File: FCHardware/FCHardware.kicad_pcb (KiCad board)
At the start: 2 copper layers, 39 x 39 mm, 51 parts, among them J2 JST-4pin, J3 JST-8pin, J4 UJ20-C-H-G-SMT-2A-P16-TR, U1 ICM-42688-P, U2 STM32F405RGTx, U3 USBLC6-2SC6, U4 AP2112K-3.3, U5 TPSM63603

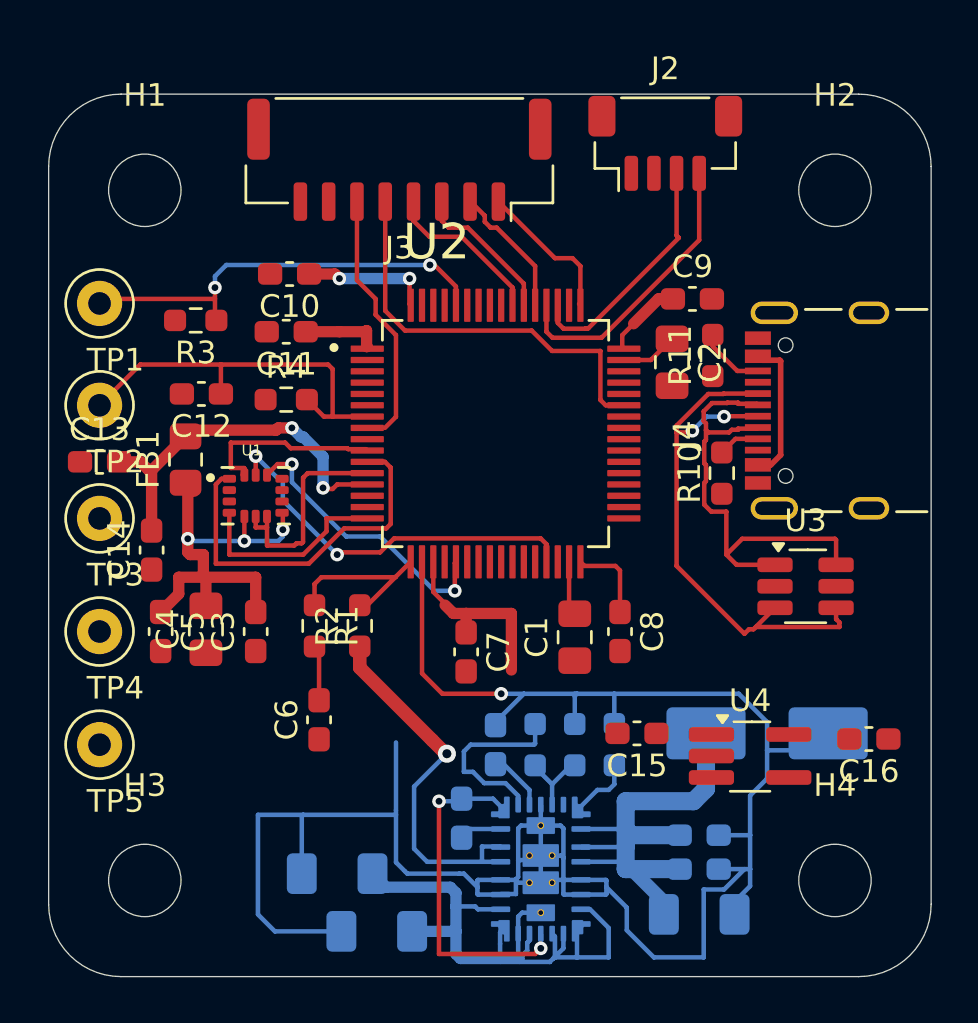
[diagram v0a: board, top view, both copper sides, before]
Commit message: Fixed USB C routing
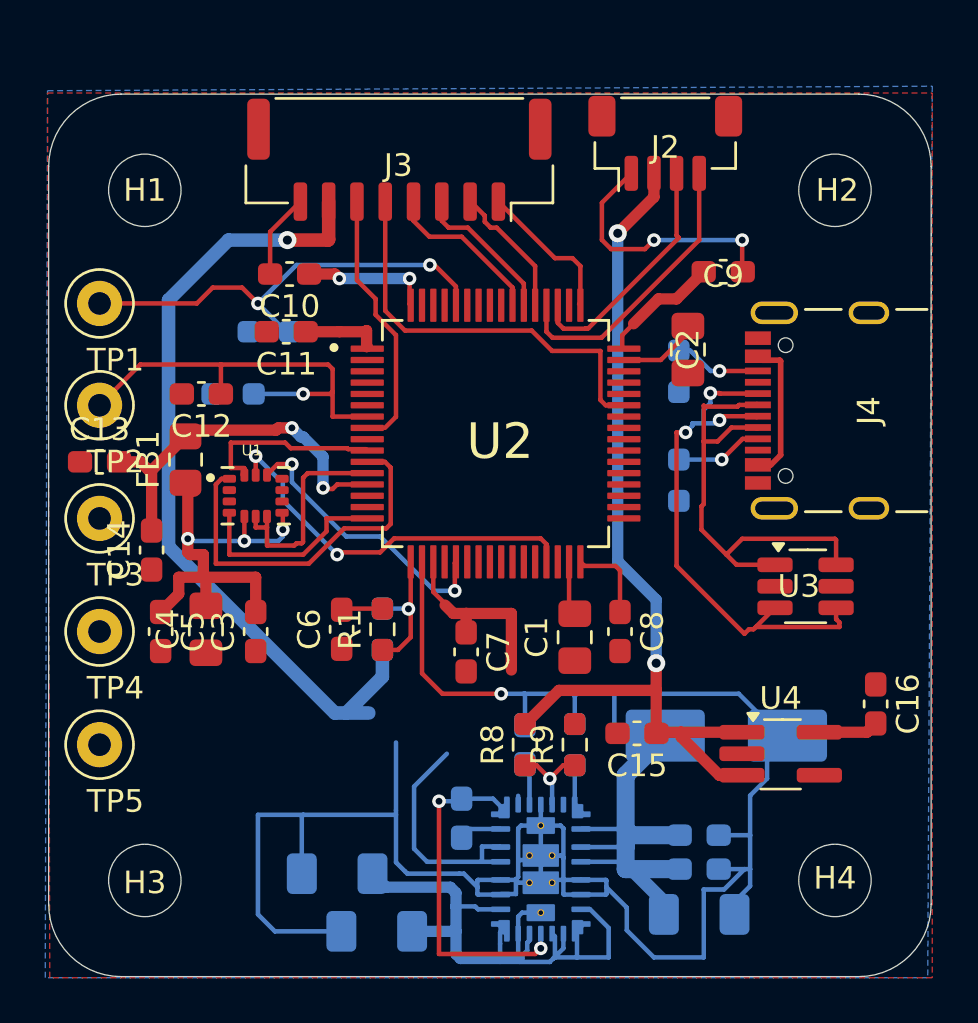
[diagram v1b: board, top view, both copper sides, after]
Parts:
- R10, R11, R2, R3, R4: moved to B.Cu
- R8, R9: moved to F.Cu
- moved C6 4.12 mm to (93.2, 103.9)
- moved R3 3.29 mm to (90.0, 90.8)
- moved R1 3.00 mm to (95.0, 103.9), turned to 90 degrees
- moved R4 2.36 mm to (88.4, 93.5)
- moved R10 1.93 mm to (108.1, 97.3)
- moved C9 1.82 mm to (110.1, 88.1)
- moved D1 1.80 mm to (110.2, 108.6)
- moved R7 1.75 mm to (103.5, 109.0)
- moved R11 1.66 mm to (108.1, 92.5)
- moved C16 1.58 mm to (116.8, 107.2), turned to -90 degrees
- moved U4 1.35 mm to (112.6, 109.4)
- moved C20 1.30 mm to (101.3, 109.0)
- moved R2 1.01 mm to (95.0, 103.9)
- moved C2 0.90 mm to (108.5, 91.5)
- moved R8 0.45 mm to (101.3, 109.0)
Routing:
- net +5V: track 37.9 -> 70.0 mm, vias 0 -> 2
- net VBAT: track 39.5 -> 66.7 mm
- net GND: track 111.8 -> 123.9 mm, vias 1 -> 3
- net +3V3: track 44.9 -> 49.4 mm
- net /NRST: track 17.5 -> 19.6 mm, vias 0 -> 1
- net Net-(J4-CC1): track 1.84 -> 3.87 mm, vias 0 -> 1
- net /V_MON: track 7.70 -> 5.97 mm, vias 0 -> 1
- net Net-(U2-VCAP_2): track 2.52 -> 3.75 mm
- net /BOOT0: track 19.2 -> 20.5 mm
- net /USB_D+: track 25.0 -> 23.9 mm, vias 2 -> 3
- net Net-(U5-RT): track 2.93 -> 2.01 mm
- net Net-(J4-CC2): track 2.96 -> 3.87 mm, vias 0 -> 1
- net Net-(U5-VCC): track 2.62 -> 1.87 mm
- net Net-(C6-Pad2): track 2.46 -> 1.82 mm
- net Net-(U5-FB): track 3.40 -> 3.88 mm, vias 0 -> 1
- added copper zone on B.Cu, net GND
- added copper zone on F.Cu, net GND
